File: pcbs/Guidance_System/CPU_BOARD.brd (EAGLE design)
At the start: 100 x 52.1 mm, 29 parts, among them J1 22-27-2081-08, J10 22-27-2081-08, J11 22-27-2081-08, J12 22-27-2081-08, J13 22-27-2081-08, J14 22-27-2081-08, J15 22-27-2041-04, J16 22-27-2041-04, J17 22-27-2021-02, J2 22-27-2021-02, J3 22-27-2041-04, J4 22-27-2041-04, J5 22-27-2081-08, J6 22-27-2021-02, J7 22-27-2081-08, J8 22-27-2021-02, J9 22-27-2021-02

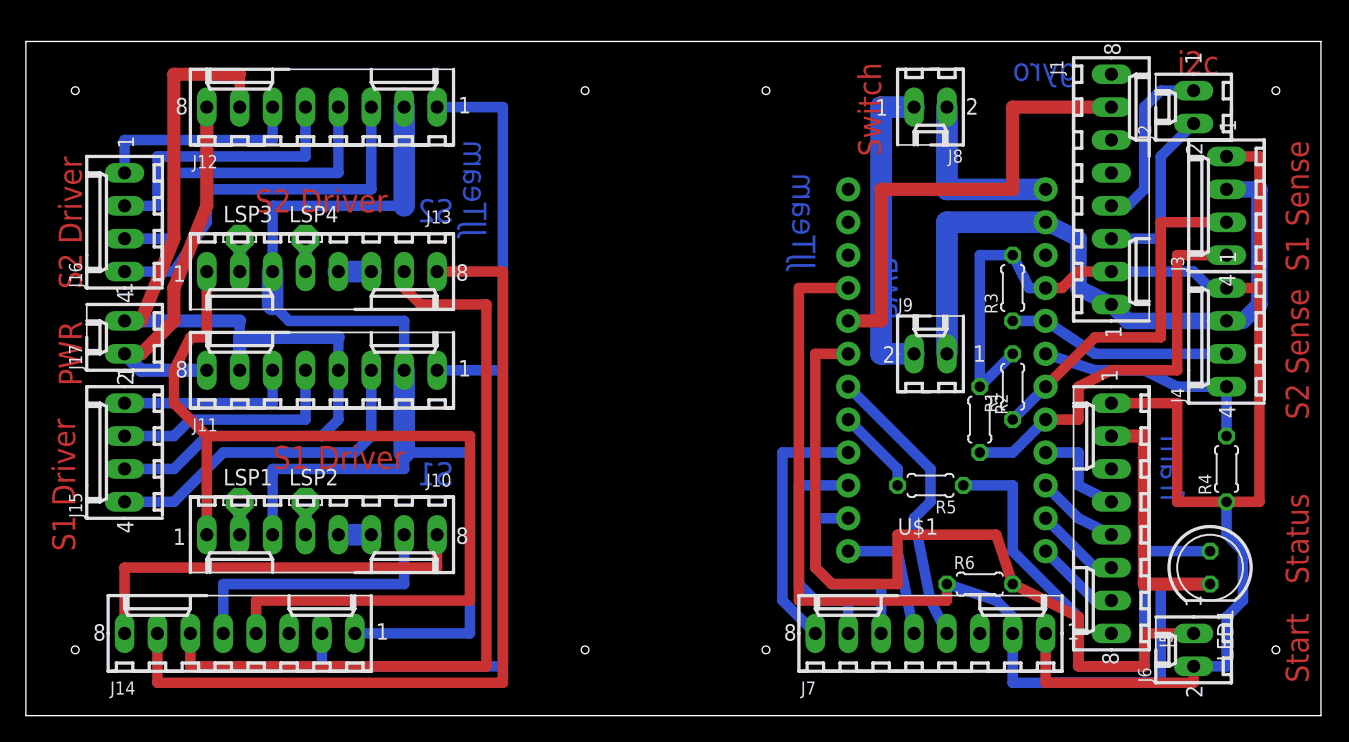
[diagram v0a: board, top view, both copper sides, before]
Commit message: * Minor adjustments
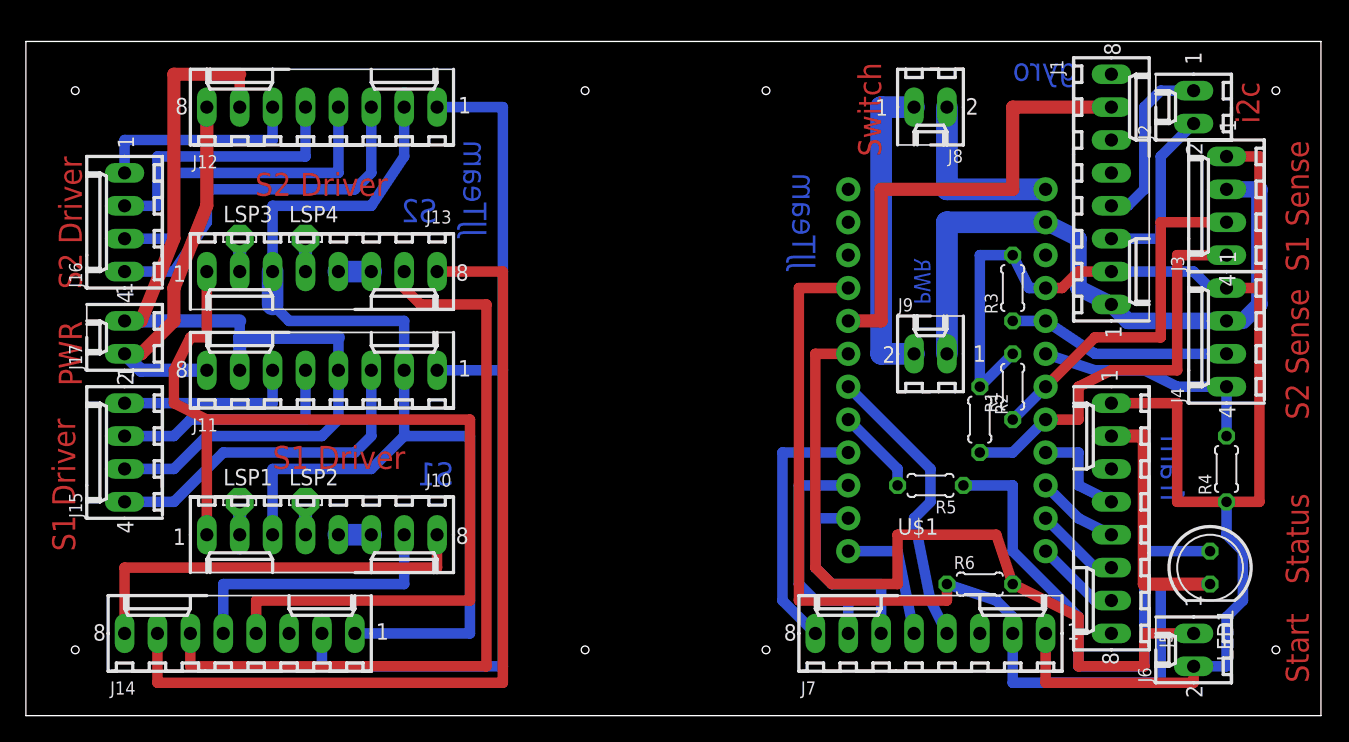
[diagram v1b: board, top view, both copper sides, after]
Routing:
- net N$32: track 90.7 -> 88.7 mm
- net N$35: track 75.0 -> 76.8 mm
- net N$44: track 30.0 -> 29.2 mm
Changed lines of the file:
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@@
 <wire x1="0" y1="77.46" x2="0" y2="25.4" width="0" layer="20"/>
 <text x="19.05" y="44.45" size="1.778" layer="1">S1 Driver</text>
-<text x="27.94" y="66.04" size="1.778" layer="1" rot="R180">S2 Driver</text>
+<text x="27.94" y="67.31" size="1.778" layer="1" rot="R180">S2 Driver</text>
 <hole x="3.81" y="30.48" drill="0.6"/>
 <hole x="57.15" y="30.48" drill="0.6"/>
@@
 <text x="99.06" y="59.69" size="1.778" layer="1" rot="R90">S1 Sense</text>
 <text x="99.06" y="48.26" size="1.778" layer="1" rot="R90">S2 Sense</text>
-<text x="67.31" y="60.96" size="1.778" layer="16" rot="MR270">PWR</text>
+<text x="68.58" y="57.15" size="1.27" layer="16" rot="MR90">PWR</text>
 <text x="66.04" y="68.58" size="1.778" layer="1" rot="R90">Switch</text>
-<text x="88.9" y="74.93" size="1.778" layer="1">i2c</text>
+<text x="95.25" y="71.12" size="1.778" layer="1" rot="R90">i2c</text>
 <text x="99.06" y="35.56" size="1.778" layer="1" rot="R90">Status</text>
 <text x="35.56" y="69.85" size="1.778" layer="16" rot="MR270">JJTeam</text>
 <text x="60.96" y="67.31" size="1.778" layer="16" rot="MR270">JJTeam</text>
 <text x="33.02" y="43.18" size="1.778" layer="16" rot="MR0">S1</text>
-<text x="33.02" y="63.5" size="1.778" layer="16" rot="MR0">S2</text>
+<text x="31.75" y="63.5" size="1.778" layer="16" rot="MR0">S2</text>
 <text x="76.2" y="76.2" size="1.778" layer="16" rot="MR180">gyro</text>
 <text x="87.63" y="41.91" size="1.778" layer="16" rot="MR90">fram</text>
@@
 <contactref element="J10" pad="3"/>
 <contactref element="J13" pad="3"/>
-<wire x1="29.21" y1="72.39" x2="29.21" y2="64.77" width="1.6764" layer="16"/>
-<wire x1="29.21" y1="64.77" x2="19.05" y2="64.77" width="0.8128" layer="16"/>
+<wire x1="29.21" y1="72.39" x2="29.21" y2="68.58" width="0.8128" layer="16"/>
+<wire x1="29.21" y1="68.58" x2="26.67" y2="64.77" width="0.8128" layer="16"/>
+<wire x1="26.67" y1="64.77" x2="19.05" y2="64.77" width="0.8128" layer="16"/>
 <wire x1="19.05" y1="64.77" x2="19.05" y2="59.69" width="0.8128" layer="16"/>
 <wire x1="19.05" y1="59.69" x2="19.05" y2="57.15" width="1.6764" layer="16"/>
@@
 <wire x1="19.05" y1="39.37" x2="19.05" y2="40.64" width="0.4064" layer="16"/>
 <wire x1="19.05" y1="40.64" x2="19.05" y2="44.45" width="0.8128" layer="16"/>
-<wire x1="19.05" y1="44.45" x2="29.21" y2="44.45" width="0.8128" layer="16"/>
-<wire x1="29.21" y1="44.45" x2="29.21" y2="45.72" width="0.8128" layer="16"/>
-<wire x1="29.21" y1="45.72" x2="29.21" y2="52.07" width="1.6764" layer="16"/>
+<wire x1="19.05" y1="44.45" x2="26.67" y2="44.45" width="0.8128" layer="16"/>
+<wire x1="26.67" y1="44.45" x2="29.21" y2="46.99" width="0.8128" layer="16"/>
+<wire x1="29.21" y1="46.99" x2="29.21" y2="52.07" width="0.8128" layer="16"/>
 <wire x1="25.4" y1="31.75" x2="34.29" y2="31.75" width="0.8128" layer="16"/>
-<wire x1="34.29" y1="31.75" x2="34.29" y2="45.72" width="0.8128" layer="16"/>
-<wire x1="34.29" y1="45.72" x2="29.21" y2="45.72" width="0.8128" layer="16"/>
+<wire x1="34.29" y1="31.75" x2="34.29" y2="46.99" width="0.8128" layer="16"/>
+<wire x1="34.29" y1="46.99" x2="29.21" y2="46.99" width="0.8128" layer="16"/>
 </signal>
 <signal name="N$33">
@@
 <wire x1="11.43" y1="59.69" x2="13.97" y2="63.5" width="0.8128" layer="16"/>
 <wire x1="13.97" y1="63.5" x2="13.97" y2="66.04" width="0.8128" layer="16"/>
-<wire x1="13.97" y1="66.04" x2="26.67" y2="66.04" width="0.8128" layer="16"/>
-<wire x1="26.67" y1="66.04" x2="26.67" y2="72.39" width="0.8128" layer="16"/>
+<wire x1="13.97" y1="66.04" x2="25.4" y2="66.04" width="0.8128" layer="16"/>
+<wire x1="25.4" y1="66.04" x2="26.67" y2="67.31" width="0.8128" layer="16"/>
+<wire x1="26.67" y1="67.31" x2="26.67" y2="72.39" width="0.8128" layer="16"/>
 </signal>
 <signal name="N$31">
@@
 <wire x1="13.97" y1="54.61" x2="12.7" y2="54.61" width="0.8128" layer="1"/>
 <wire x1="12.7" y1="54.61" x2="11.43" y2="52.07" width="0.8128" layer="1"/>
-<wire x1="13.97" y1="46.99" x2="11.43" y2="49.53" width="0.8128" layer="1"/>
+<wire x1="13.97" y1="48.26" x2="11.43" y2="49.53" width="0.8128" layer="1"/>
 <wire x1="11.43" y1="49.53" x2="11.43" y2="52.07" width="0.8128" layer="1"/>
-<wire x1="13.97" y1="39.37" x2="13.97" y2="46.99" width="0.8128" layer="1"/>
-<wire x1="13.97" y1="46.99" x2="34.29" y2="46.99" width="0.8128" layer="1"/>
-<wire x1="34.29" y1="46.99" x2="34.29" y2="34.29" width="0.8128" layer="1"/>
+<wire x1="13.97" y1="39.37" x2="13.97" y2="48.26" width="0.8128" layer="1"/>
+<wire x1="13.97" y1="48.26" x2="34.29" y2="48.26" width="0.8128" layer="1"/>
+<wire x1="34.29" y1="48.26" x2="34.29" y2="34.29" width="0.8128" layer="1"/>
 <wire x1="34.29" y1="34.29" x2="17.78" y2="34.29" width="0.8128" layer="1"/>
 <wire x1="17.78" y1="34.29" x2="17.78" y2="31.75" width="0.8128" layer="1"/>
@@
 </signal>
 </signals>
+<errors>
+</errors>
 </board>
 </drawing>
